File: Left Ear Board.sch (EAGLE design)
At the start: 5 parts

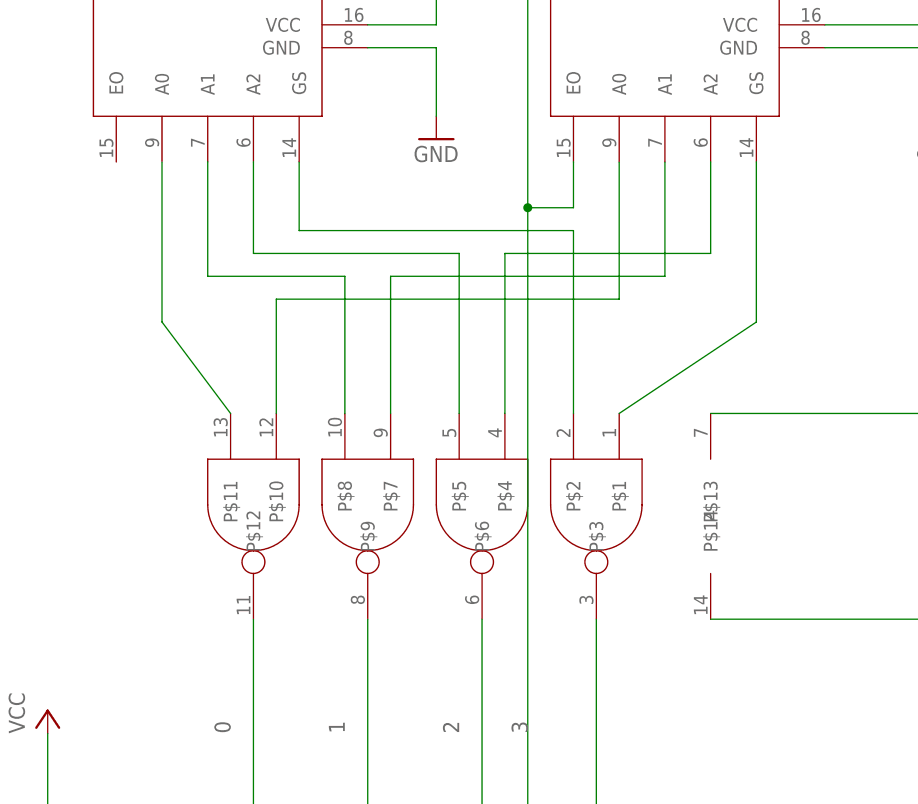
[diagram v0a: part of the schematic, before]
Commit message: Worked on board schematic
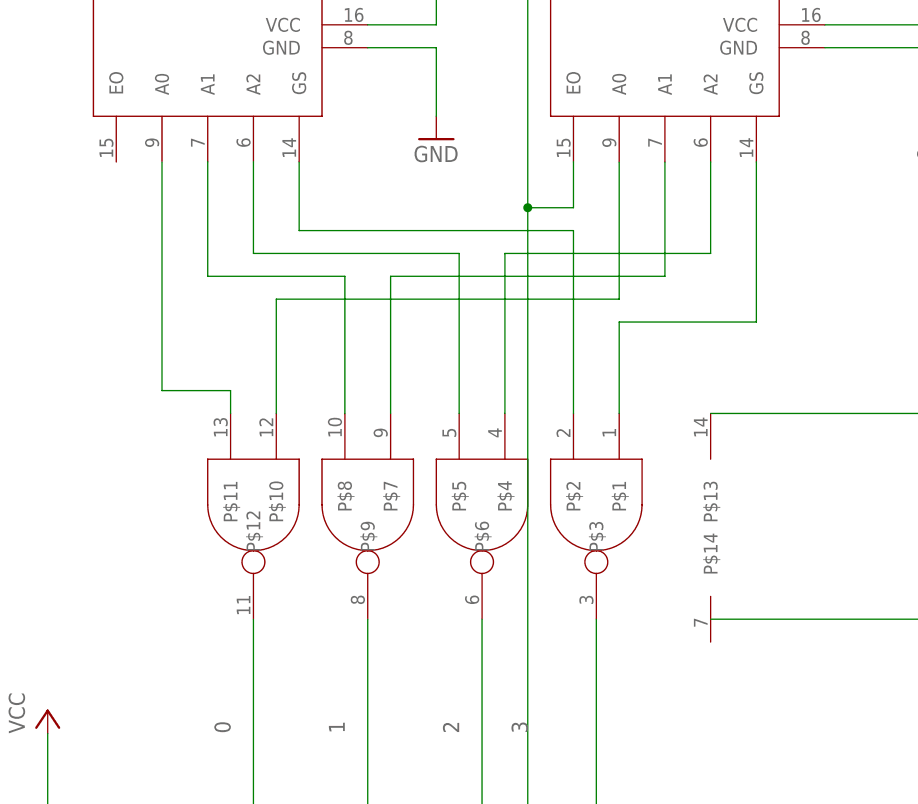
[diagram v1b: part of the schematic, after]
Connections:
- net GND: no longer U$4.P$14
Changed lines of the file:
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@@
 <part name="GND3" library="supply1" library_urn="urn:adsk.eagle:library:371" deviceset="GND" device=""/>
 <part name="GND4" library="supply1" library_urn="urn:adsk.eagle:library:371" deviceset="GND" device=""/>
-<part name="U$4" library="FormE" deviceset="QUAD_NAND" device=""/>
 <part name="P+3" library="supply1" library_urn="urn:adsk.eagle:library:371" deviceset="VCC" device=""/>
 <part name="GND5" library="supply1" library_urn="urn:adsk.eagle:library:371" deviceset="GND" device=""/>
@@
 <part name="P+4" library="supply1" library_urn="urn:adsk.eagle:library:371" deviceset="VCC" device=""/>
 <part name="GND6" library="supply1" library_urn="urn:adsk.eagle:library:371" deviceset="GND" device=""/>
+<part name="U$4" library="FormE" deviceset="QUAD_NAND" device=""/>
 </parts>
 <sheets>
@@
 <instance part="GND3" gate="1" x="187.96" y="33.02"/>
 <instance part="GND4" gate="1" x="165.1" y="96.52"/>
-<instance part="U$4" gate="G$1" x="137.16" y="-7.62" rot="R270"/>
 <instance part="P+3" gate="VCC" x="190.5" y="7.62"/>
 <instance part="GND5" gate="1" x="190.5" y="-35.56"/>
@@
 <instance part="P+4" gate="VCC" x="88.9" y="-30.48"/>
 <instance part="GND6" gate="1" x="88.9" y="-73.66"/>
+<instance part="U$4" gate="G$1" x="132.08" y="7.62" rot="R270"/>
 </instances>
 <busses>
@@
 </segment>
 <segment>
+<pinref part="SV1" gate="1" pin="8"/>
+<wire x1="86.36" y1="-45.72" x2="88.9" y2="-45.72" width="0.1524" layer="91"/>
+<wire x1="88.9" y1="-45.72" x2="88.9" y2="-33.02" width="0.1524" layer="91"/>
+<pinref part="P+4" gate="VCC" pin="VCC"/>
+</segment>
+<segment>
 <pinref part="U$4" gate="G$1" pin="P$13"/>
 <pinref part="P+3" gate="VCC" pin="VCC"/>
 <wire x1="162.56" y1="2.54" x2="190.5" y2="2.54" width="0.1524" layer="91"/>
 <wire x1="190.5" y1="2.54" x2="190.5" y2="5.08" width="0.1524" layer="91"/>
-</segment>
-<segment>
-<pinref part="SV1" gate="1" pin="8"/>
-<wire x1="86.36" y1="-45.72" x2="88.9" y2="-45.72" width="0.1524" layer="91"/>
-<wire x1="88.9" y1="-45.72" x2="88.9" y2="-33.02" width="0.1524" layer="91"/>
-<pinref part="P+4" gate="VCC" pin="VCC"/>
 </segment>
 </net>
@@
 </segment>
 <segment>
-<pinref part="U$4" gate="G$1" pin="P$14"/>
 <pinref part="GND5" gate="1" pin="GND"/>
 <wire x1="162.56" y1="-20.32" x2="190.5" y2="-20.32" width="0.1524" layer="91"/>
@@
 <segment>
 <pinref part="U$2" gate="G$1" pin="A0"/>
-<wire x1="101.6" y1="30.48" x2="101.6" y2="12.7" width="0.1524" layer="91"/>
-<wire x1="101.6" y1="12.7" x2="109.22" y2="2.54" width="0.1524" layer="91"/>
+<wire x1="101.6" y1="30.48" x2="101.6" y2="5.08" width="0.1524" layer="91"/>
 <pinref part="U$4" gate="G$1" pin="P$11"/>
+<wire x1="101.6" y1="5.08" x2="109.22" y2="5.08" width="0.1524" layer="91"/>
+<wire x1="109.22" y1="5.08" x2="109.22" y2="2.54" width="0.1524" layer="91"/>
 </segment>
 </net>
@@
 <segment>
 <pinref part="U$3" gate="G$1" pin="GS"/>
+<wire x1="167.64" y1="30.48" x2="167.64" y2="12.7" width="0.1524" layer="91"/>
 <pinref part="U$4" gate="G$1" pin="P$1"/>
-<wire x1="167.64" y1="30.48" x2="167.64" y2="12.7" width="0.1524" layer="91"/>
-<wire x1="167.64" y1="12.7" x2="152.4" y2="2.54" width="0.1524" layer="91"/>
+<wire x1="152.4" y1="2.54" x2="152.4" y2="12.7" width="0.1524" layer="91"/>
+<wire x1="152.4" y1="12.7" x2="167.64" y2="12.7" width="0.1524" layer="91"/>
 </segment>
 </net>
 <net name="2" class="0">
 <segment>
-<pinref part="U$4" gate="G$1" pin="P$6"/>
 <label x="134.62" y="-33.02" size="1.778" layer="95" rot="R90"/>
 <pinref part="SV1" gate="1" pin="5"/>
 <wire x1="86.36" y1="-53.34" x2="137.16" y2="-53.34" width="0.1524" layer="91"/>
 <wire x1="137.16" y1="-53.34" x2="137.16" y2="-20.32" width="0.1524" layer="91"/>
+<pinref part="U$4" gate="G$1" pin="P$6"/>
 </segment>
 </net>
 <net name="1" class="0">
 <segment>
-<pinref part="U$4" gate="G$1" pin="P$9"/>
 <label x="121.92" y="-33.02" size="1.778" layer="95" rot="R90"/>
 <pinref part="SV1" gate="1" pin="6"/>
 <wire x1="86.36" y1="-50.8" x2="124.46" y2="-50.8" width="0.1524" layer="91"/>
 <wire x1="124.46" y1="-50.8" x2="124.46" y2="-20.32" width="0.1524" layer="91"/>
+<pinref part="U$4" gate="G$1" pin="P$9"/>
 </segment>
 </net>
 <net name="0" class="0">
 <segment>
-<pinref part="U$4" gate="G$1" pin="P$12"/>
 <wire x1="111.76" y1="-20.32" x2="111.76" y2="-48.26" width="0.1524" layer="91"/>
 <label x="109.22" y="-33.02" size="1.778" layer="95" rot="R90"/>
 <pinref part="SV1" gate="1" pin="7"/>
 <wire x1="86.36" y1="-48.26" x2="111.76" y2="-48.26" width="0.1524" layer="91"/>
+<pinref part="U$4" gate="G$1" pin="P$12"/>
 </segment>
 </net>
 <net name="N$21" class="0">
 <segment>
-<pinref part="U$4" gate="G$1" pin="P$3"/>
 <pinref part="SV1" gate="1" pin="3"/>
 <wire x1="86.36" y1="-58.42" x2="149.86" y2="-58.42" width="0.1524" layer="91"/>
 <wire x1="149.86" y1="-58.42" x2="149.86" y2="-20.32" width="0.1524" layer="91"/>
-</segment>
-</net>
+<pinref part="U$4" gate="G$1" pin="P$3"/>
+</segment>
+</net>
